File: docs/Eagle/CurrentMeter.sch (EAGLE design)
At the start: 10 parts

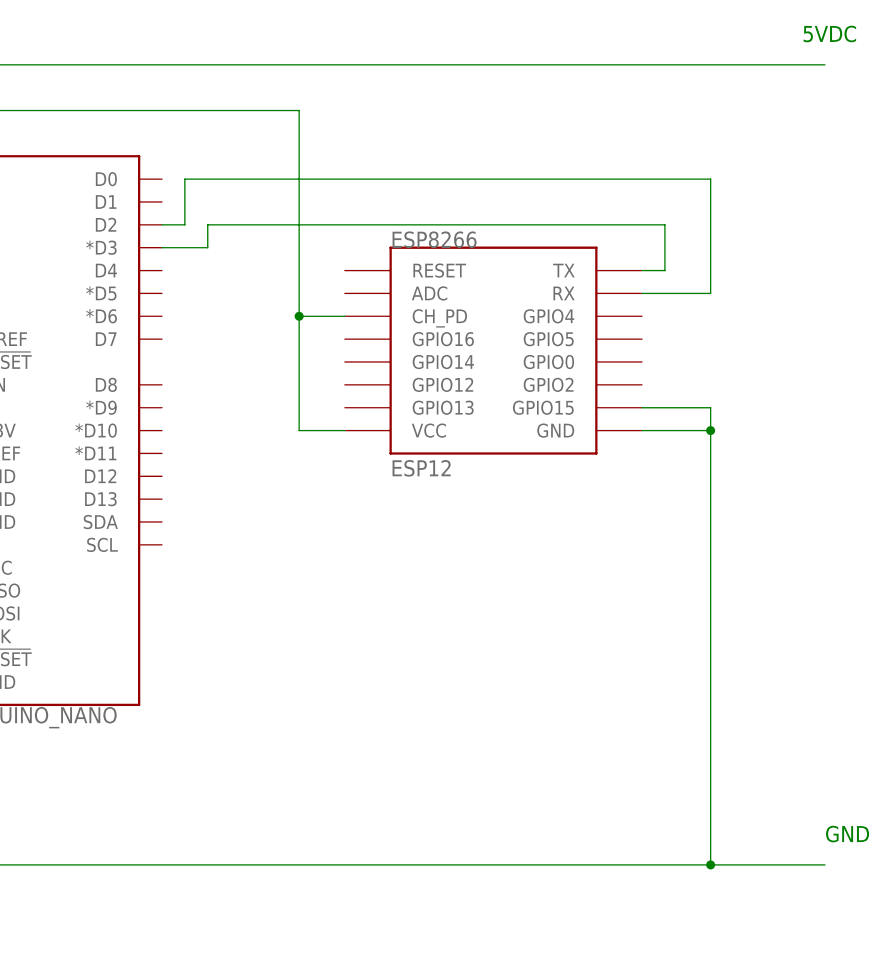
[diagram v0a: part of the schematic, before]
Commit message: schematics finalized
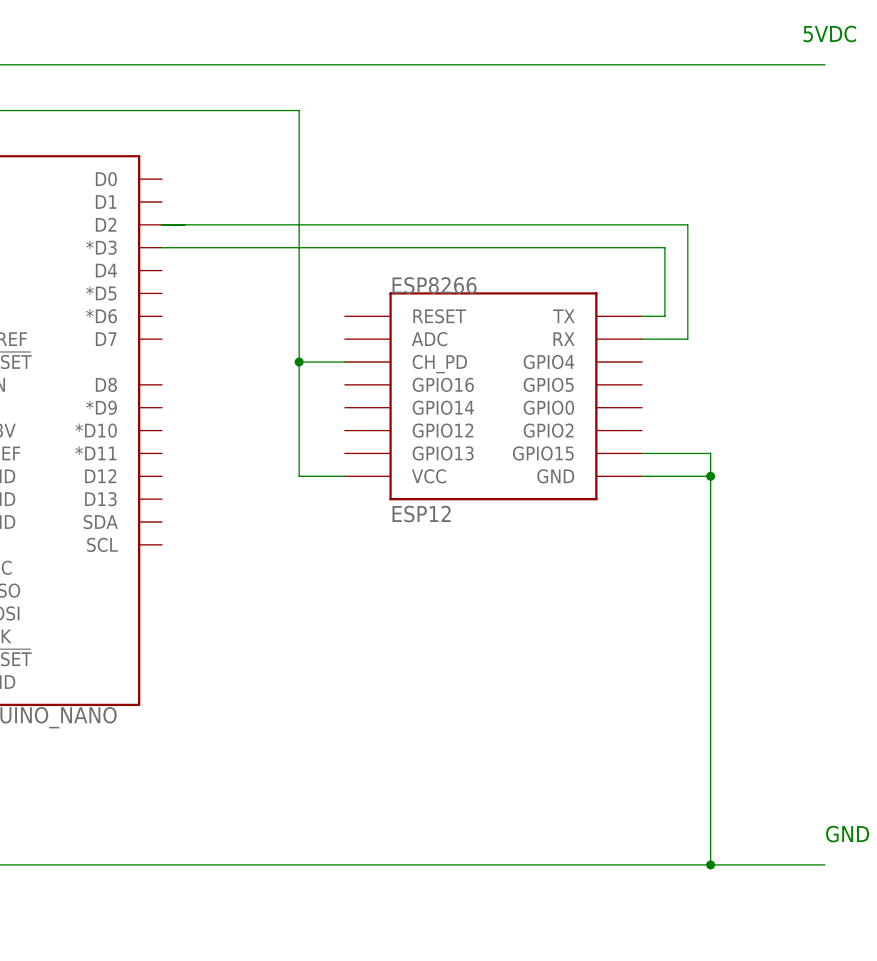
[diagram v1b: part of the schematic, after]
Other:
- moved on the sheet: ESP8266
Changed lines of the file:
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@@
 <?xml version="1.0" encoding="utf-8"?>
 <!DOCTYPE eagle SYSTEM "eagle.dtd">
-<eagle version="9.4.1">
+<eagle version="9.4.2">
 <drawing>
 <settings>
@@
 <attribute name="VALUE" x="87.122" y="31.75" size="1.778" layer="96" rot="R90"/>
 </instance>
-<instance part="ESP8266" gate="G$1" x="180.34" y="71.12" smashed="yes">
-<attribute name="NAME" x="167.64" y="81.28" size="1.778" layer="95"/>
-<attribute name="VALUE" x="167.64" y="55.88" size="1.778" layer="96"/>
+<instance part="ESP8266" gate="G$1" x="180.34" y="66.04" smashed="yes">
+<attribute name="NAME" x="167.64" y="76.2" size="1.778" layer="95"/>
+<attribute name="VALUE" x="167.64" y="50.8" size="1.778" layer="96"/>
 </instance>
 </instances>
@@
 <junction x="111.76" y="12.7"/>
 <wire x1="215.9" y1="12.7" x2="203.2" y2="12.7" width="0.1524" layer="91"/>
-<wire x1="203.2" y1="12.7" x2="203.2" y2="60.96" width="0.1524" layer="91"/>
+<wire x1="203.2" y1="12.7" x2="203.2" y2="55.88" width="0.1524" layer="91"/>
 <junction x="203.2" y="12.7"/>
 <pinref part="ESP8266" gate="G$1" pin="GND"/>
-<wire x1="203.2" y1="60.96" x2="195.58" y2="60.96" width="0.1524" layer="91"/>
-<wire x1="203.2" y1="60.96" x2="203.2" y2="63.5" width="0.1524" layer="91"/>
-<junction x="203.2" y="60.96"/>
+<wire x1="203.2" y1="55.88" x2="195.58" y2="55.88" width="0.1524" layer="91"/>
+<wire x1="203.2" y1="55.88" x2="203.2" y2="58.42" width="0.1524" layer="91"/>
+<junction x="203.2" y="55.88"/>
 <pinref part="ESP8266" gate="G$1" pin="GPIO15"/>
-<wire x1="203.2" y1="63.5" x2="195.58" y2="63.5" width="0.1524" layer="91"/>
+<wire x1="203.2" y1="58.42" x2="195.58" y2="58.42" width="0.1524" layer="91"/>
 </segment>
 </net>
@@
 <wire x1="114.3" y1="60.96" x2="114.3" y2="96.52" width="0.1524" layer="91"/>
 <wire x1="114.3" y1="96.52" x2="157.48" y2="96.52" width="0.1524" layer="91"/>
-<wire x1="157.48" y1="96.52" x2="157.48" y2="73.66" width="0.1524" layer="91"/>
+<wire x1="157.48" y1="96.52" x2="157.48" y2="68.58" width="0.1524" layer="91"/>
 <pinref part="ESP8266" gate="G$1" pin="VCC"/>
-<wire x1="157.48" y1="73.66" x2="157.48" y2="60.96" width="0.1524" layer="91"/>
-<wire x1="157.48" y1="60.96" x2="162.56" y2="60.96" width="0.1524" layer="91"/>
+<wire x1="157.48" y1="68.58" x2="157.48" y2="55.88" width="0.1524" layer="91"/>
+<wire x1="157.48" y1="55.88" x2="162.56" y2="55.88" width="0.1524" layer="91"/>
 <pinref part="ESP8266" gate="G$1" pin="CH_PD"/>
-<wire x1="162.56" y1="73.66" x2="157.48" y2="73.66" width="0.1524" layer="91"/>
-<junction x="157.48" y="73.66"/>
+<wire x1="162.56" y1="68.58" x2="157.48" y2="68.58" width="0.1524" layer="91"/>
+<junction x="157.48" y="68.58"/>
 </segment>
 </net>
@@
 <segment>
 <pinref part="B1" gate="G$1" pin="D2"/>
-<wire x1="142.24" y1="83.82" x2="144.78" y2="83.82" width="0.1524" layer="91"/>
-<wire x1="144.78" y1="83.82" x2="144.78" y2="88.9" width="0.1524" layer="91"/>
-<wire x1="144.78" y1="88.9" x2="203.2" y2="88.9" width="0.1524" layer="91"/>
-<wire x1="203.2" y1="88.9" x2="203.2" y2="76.2" width="0.1524" layer="91"/>
+<wire x1="144.78" y1="83.82" x2="142.24" y2="83.82" width="0.1524" layer="91"/>
+<wire x1="142.24" y1="83.82" x2="200.66" y2="83.82" width="0.1524" layer="91"/>
+<wire x1="200.66" y1="83.82" x2="200.66" y2="71.12" width="0.1524" layer="91"/>
 <pinref part="ESP8266" gate="G$1" pin="RX"/>
-<wire x1="203.2" y1="76.2" x2="195.58" y2="76.2" width="0.1524" layer="91"/>
+<wire x1="200.66" y1="71.12" x2="195.58" y2="71.12" width="0.1524" layer="91"/>
 </segment>
 </net>
@@
 <segment>
 <pinref part="B1" gate="G$1" pin="*D3"/>
-<wire x1="142.24" y1="81.28" x2="147.32" y2="81.28" width="0.1524" layer="91"/>
-<wire x1="147.32" y1="81.28" x2="147.32" y2="83.82" width="0.1524" layer="91"/>
-<wire x1="147.32" y1="83.82" x2="198.12" y2="83.82" width="0.1524" layer="91"/>
+<wire x1="142.24" y1="81.28" x2="198.12" y2="81.28" width="0.1524" layer="91"/>
 <pinref part="ESP8266" gate="G$1" pin="TX"/>
-<wire x1="198.12" y1="83.82" x2="198.12" y2="78.74" width="0.1524" layer="91"/>
-<wire x1="198.12" y1="78.74" x2="195.58" y2="78.74" width="0.1524" layer="91"/>
-</segment>
-</net>
+<wire x1="198.12" y1="81.28" x2="198.12" y2="73.66" width="0.1524" layer="91"/>
+<wire x1="198.12" y1="73.66" x2="195.58" y2="73.66" width="0.1524" layer="91"/>
+</segment>
+</net>
